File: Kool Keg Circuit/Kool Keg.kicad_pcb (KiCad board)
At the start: 2 copper layers, 84 parts, among them J1 Power, J2 Scale Header, J3 IR Header, J4 Flowmeter, J5 OLED, J6 Solenoid Conn, J7 USB_B_Micro, Q1 2N3905, Q2 2N3906, Q3 BC818, Q4 BC818, SW1 SW, SW2 SW, SW3 SW, SW4 SW_Push, SW5 SW_EN, U1 LM1117-ADJ, U2 TPS562207, U3 74LVC3G14, U4 HX711, U5 24LC256, U6 MPQ6610GS, U7 CP2102N, U8 ESP32-WROOM-32D

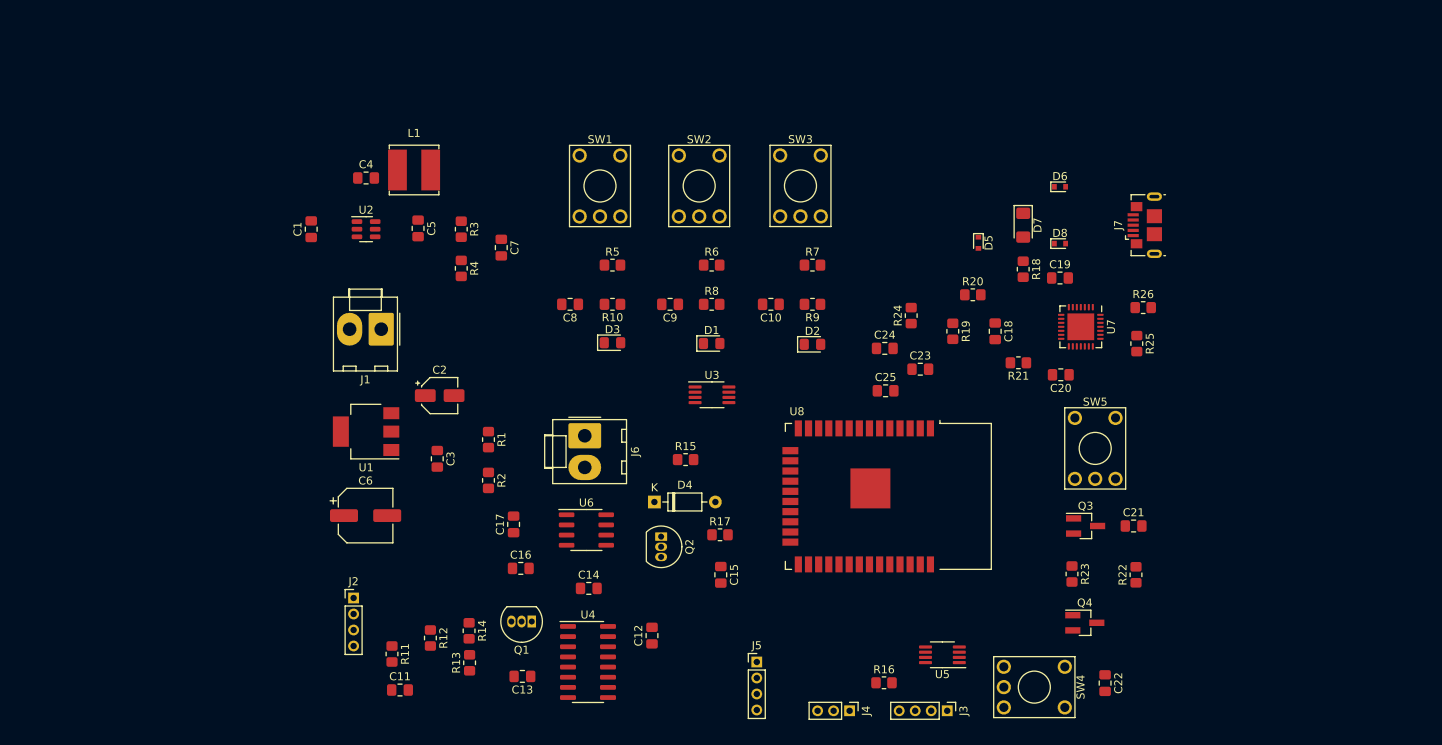
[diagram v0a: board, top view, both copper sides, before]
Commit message: PCB Layout
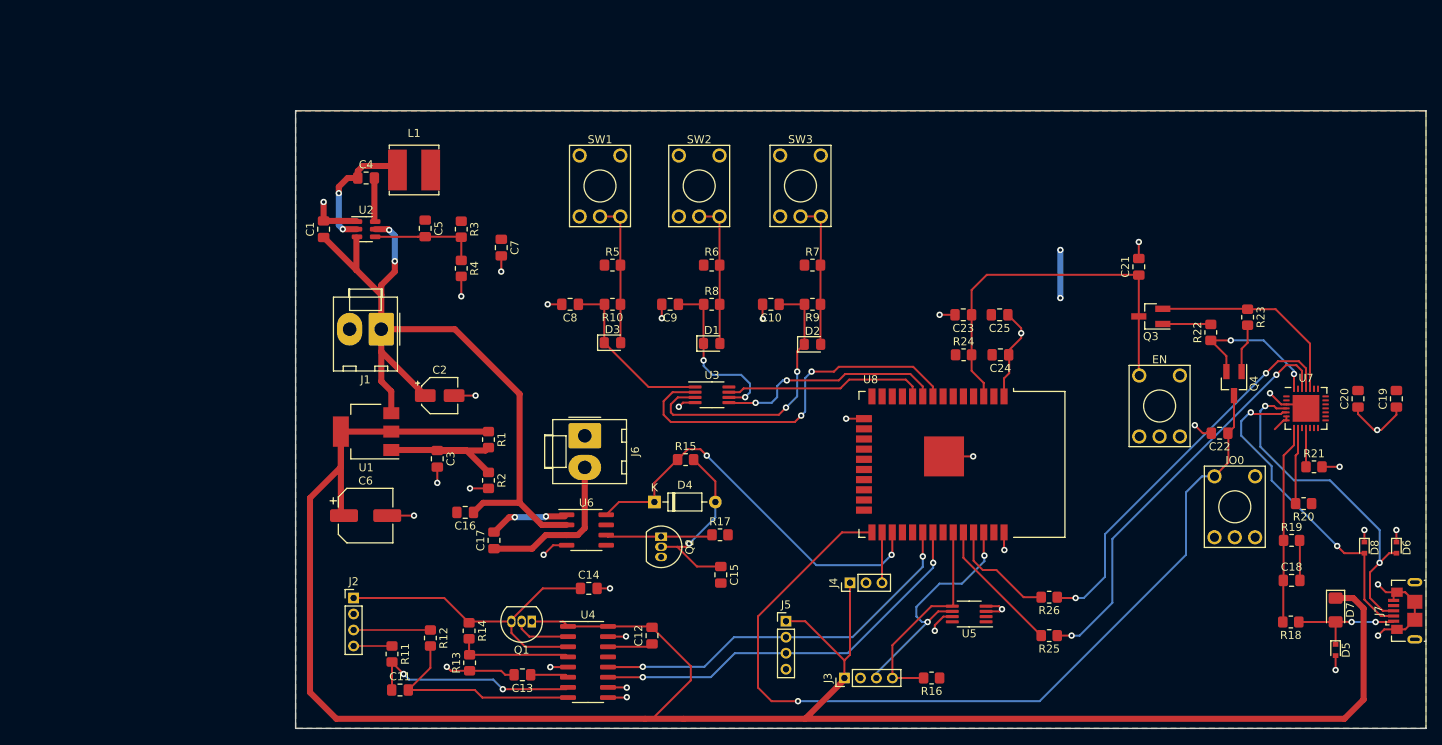
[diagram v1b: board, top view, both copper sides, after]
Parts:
- EN: renamed from SW5; value SW_EN -> SW_Push
- moved D5 67.7 mm to (225.7, 119.8)
- moved D7 62.0 mm to (225.7, 114.8)
- moved D6 61.7 mm to (233.3, 107.0), turned to -90 degrees
- moved J7 58.2 mm to (234.4, 114.9)
- moved R18 55.4 mm to (220.1, 116.3), turned to 180 degrees
- moved D8 53.8 mm to (229.3, 107.0), turned to -90 degrees
- moved R19 49.8 mm to (220.2, 106.1), turned to 0 degrees
- moved R20 48.9 mm to (221.7, 101.5), turned to 180 degrees
- moved C18 48.4 mm to (220.2, 111.1), turned to 0 degrees
- moved C19 44.7 mm to (233.3, 88.4), turned to 90 degrees
- moved R21 39.2 mm to (223.0, 96.9), turned to 0 degrees
- moved R23 38.9 mm to (214.7, 78.2)
- moved R25 38.1 mm to (189.9, 118.0), turned to 180 degrees
- moved R26 38.1 mm to (189.9, 113.2), turned to 180 degrees
- moved C20 37.3 mm to (228.5, 88.4), turned to 90 degrees
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- renumbered SW4 to IO0
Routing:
- net +5V: track 0.00 -> 273.8 mm
- net GND: track 0.00 -> 126.6 mm, vias 0 -> 35
- net /MCU Subsystem/IO0: track 0.00 -> 112.6 mm, vias 0 -> 1
- net +12V: track 0.00 -> 99.7 mm, vias 0 -> 2
- net /MCU Subsystem/TXD: track 0.00 -> 51.8 mm, vias 0 -> 2
- net /MCU Subsystem/I2C1_SCL: track 0.00 -> 50.7 mm, vias 0 -> 2
- net /MCU Subsystem/SOLENOID_GPIO: track 0.00 -> 49.9 mm, vias 0 -> 2
- net /MCU Subsystem/RXD: track 0.00 -> 49.4 mm, vias 0 -> 2
- net /MCU Subsystem/I2C1_SDA: track 0.00 -> 48.8 mm, vias 0 -> 2
- net /MCU Subsystem/EN: track 0.00 -> 48.2 mm
- net /MCU Subsystem/DEC: track 0.00 -> 47.7 mm, vias 0 -> 2
- net /MCU Subsystem/USB_DP: track 0.00 -> 42.5 mm, vias 0 -> 2
- net /MCU Subsystem/USB_DN: track 0.00 -> 40.9 mm, vias 0 -> 2
- net /Sensor Subsystem/E+: track 0.00 -> 40.0 mm
- net Net-(C10-Pad1): track 0.00 -> 36.3 mm, vias 0 -> 2
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- added copper zone on F.Cu, net +3.3V
- added copper zone on B.Cu, net GND
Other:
- board outline added: 141.3 x 77.2 mm

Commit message: PCB
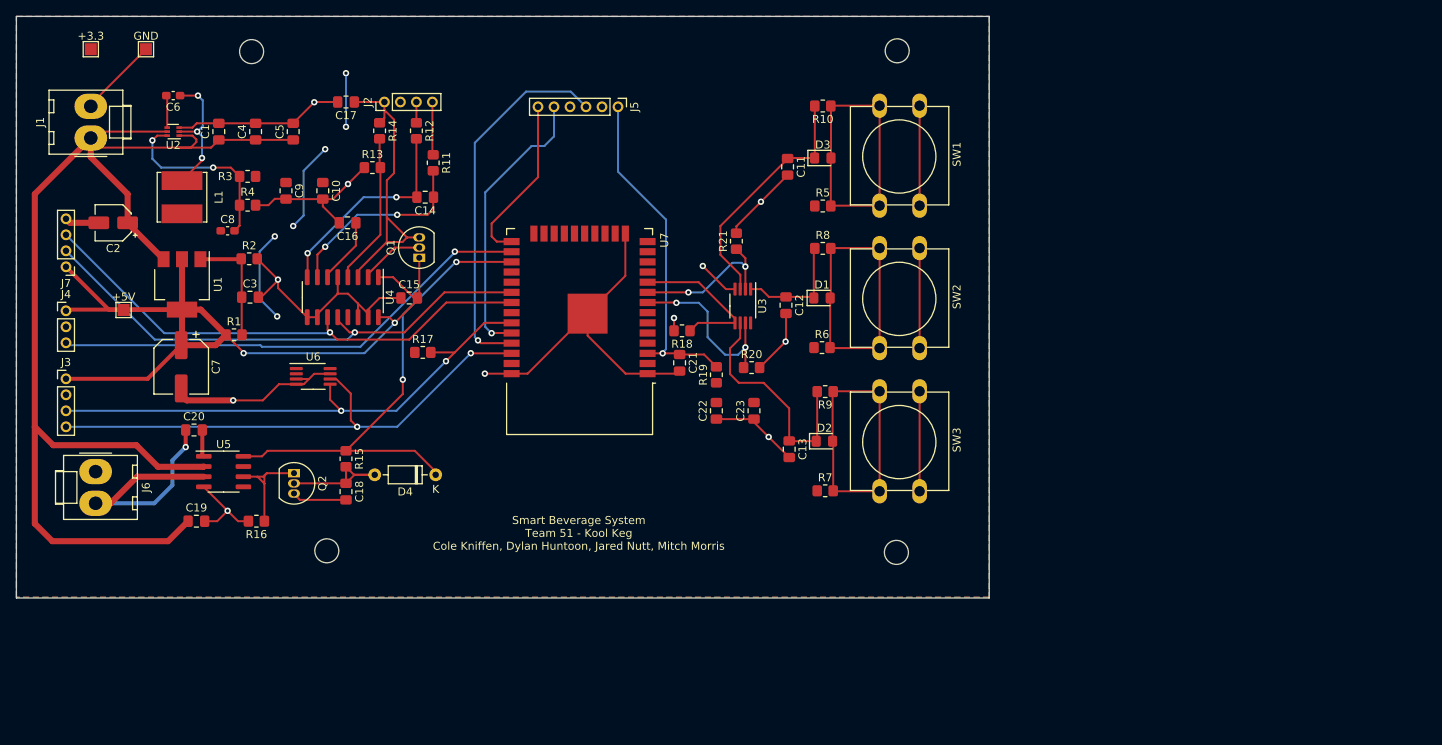
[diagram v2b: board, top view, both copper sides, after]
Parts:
- removed C24: 22uF, Capacitor_SMD:C_0805_2012Metric_Pad1.18x1.45mm_HandSolder
- removed C25: 0.1uF, Capacitor_SMD:C_0805_2012Metric_Pad1.18x1.45mm_HandSolder
- removed D5, D6, D8: LED, Diode_SMD:D_SOD-523
- removed D7: 1N5819, Diode_SMD:D_1206_3216Metric_Pad1.42x1.75mm_HandSolder
- removed EN, IO0: SW_Push, Button_Switch_THT:KSA_Tactile_SPST
- removed Q3, Q4: BC818, Package_TO_SOT_SMD:SOT-23_Handsoldering-BC808-25LT1g
- removed R22, R23, R24: 10k, Resistor_SMD:R_0805_2012Metric_Pad1.20x1.40mm_HandSolder
- removed R25, R26: 0R, Resistor_SMD:R_0805_2012Metric_Pad1.20x1.40mm_HandSolder
- removed U8: ESP32-WROOM-32D, RF_Module:ESP32-WROOM-32
- added +3.3: TestPoint_Pad_1.5x1.5mm, TestPoint:TestPoint_Pad_1.5x1.5mm, F.Cu at (70.1, 44.7)
- added +5V: TestPoint_Pad_1.5x1.5mm, TestPoint:TestPoint_Pad_1.5x1.5mm, F.Cu at (74.2, 77.3)
- added GND: TestPoint_Pad_1.5x1.5mm, TestPoint:TestPoint_Pad_1.5x1.5mm, F.Cu at (77.0, 44.7)
- added REF**: MountingHole_3mm, MountingHole:MountingHole_3mm, F.Cu at (99.6, 107.4)
- added REF**: MountingHole_3mm, MountingHole:MountingHole_3mm, F.Cu at (170.9, 44.9)
- added REF**: MountingHole_3mm, MountingHole:MountingHole_3mm, F.Cu at (170.8, 107.6)
- added REF**: MountingHole_3mm, MountingHole:MountingHole_3mm, F.Cu at (90.2, 45.0)
- C1: value 22uf -> 100nF
- C10, C9: value 0.1uF -> 22uF
- C12, C14: value 10uF -> 0.1uF
- C15: value 2.2uF -> 10uF
- C16: value .1uF -> 0.1uF
- C17: value 100 nF -> 10uF
- C18: value 10uF -> 2.2uF
- C19: value 4.7 uF -> .1uF
- C20: value 0.1 uF -> 100 nF
- C22: value 1n -> 22uF
- C23: value 1n -> 0.1uF
- C3: value 56nF -> 68nF
- C4: value .1uF -> 10uF
- C5: value 22pF -> 10uF
- C6: value 100uF -> .1uF; footprint Capacitor_SMD:CP_Elec_6.3x5.8 -> Capacitor_SMD:C_0603_1608Metric_Pad1.08x0.95mm_HandSolder
- C7: value 44uF -> 100uF; footprint Capacitor_SMD:C_0805_2012Metric_Pad1.18x1.45mm_HandSolder -> Capacitor_SMD:CP_Elec_6.3x5.8
- C8: value 0.1uF -> 56pF; footprint Capacitor_SMD:C_0805_2012Metric_Pad1.18x1.45mm_HandSolder -> Capacitor_SMD:C_0603_1608Metric_Pad1.08x0.95mm_HandSolder
- J3: value IR Header -> IR
- J4: value Flowmeter -> Flow
- J5: value OLED -> Prog; footprint Connector_PinHeader_2.00mm:PinHeader_1x04_P2.00mm_Vertical -> Connector_PinHeader_2.00mm:PinHeader_1x06_P2.00mm_Vertical
- J6: value Solenoid Conn -> Soloenoid
- J7: value USB_B_Micro -> OLED; footprint Connector_USB:USB_Micro-B_GCT_USB3076-30-A -> Connector_PinHeader_2.00mm:PinHeader_1x04_P2.00mm_Vertical
- R18: value 22.1k -> 10k
- R19: value 47.5k -> 10k
- R20: value 2k -> 10k
- SW1, SW2, SW3: value SW -> SW_MEC_5G; footprint Button_Switch_THT:KSA_Tactile_SPST -> Button_Switch_THT:SW_PUSH-12mm
- U2: footprint Package_TO_SOT_SMD:SOT-23-6 -> Package_TO_SOT_SMD:SOT-563
- U5: value 24LC256 -> 946-MPQ6610GS-AEC1-P; footprint Package_SO:MSOP-8_3x3mm_P0.65mm -> Package_SO:SOIC-8_3.9x4.9mm_P1.27mm
- U6: value MPQ6610GS -> 24LC256-I/MS; footprint Package_SO:SOIC-8_3.9x4.9mm_P1.27mm -> Package_SO:MSOP-8_3x3mm_P0.65mm
- U7: value CP2102N -> ESP32-WROOM-32D; footprint Package_DFN_QFN:QFN-28-1EP_5x5mm_P0.5mm_EP3.35x3.35mm -> RF_Module:ESP32-WROOM-32
- moved J7 172.8 mm to (67.0, 71.9), turned to 180 degrees
- moved C19 150.8 mm to (83.3, 103.7), turned to 0 degrees
- moved C20 145.6 mm to (83.0, 92.3), turned to 0 degrees
- moved C18 118.7 mm to (102.0, 100.0), turned to -90 degrees
- moved J3 104.2 mm to (67.0, 85.9), turned to 0 degrees
- moved J4 103.7 mm to (67.0, 77.4), turned to 0 degrees
- moved U5 94.9 mm to (86.7, 97.5), turned to 0 degrees
- moved U7 91.7 mm to (131.2, 77.0), turned to 180 degrees
- moved R16 86.6 mm to (90.8, 103.7)
- moved R18 84.4 mm to (144.0, 79.9)
- moved C11 81.4 mm to (157.2, 59.4), turned to -90 degrees
- moved R21 77.5 mm to (150.8, 68.7), turned to 90 degrees
- moved R19 74.8 mm to (148.3, 85.4), turned to 90 degrees
- moved R20 71.1 mm to (152.7, 84.5), turned to 0 degrees
- moved J5 67.6 mm to (136.0, 51.9), turned to -90 degrees
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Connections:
- C10 pad 1: Net-(C10-Pad1) -> +3.3V
- C11 pad 2: Net-(C11-Pad2) -> GND
- C12 pad 1: GND -> Net-(C12-Pad1)
- C12 pad 2: +5V -> GND
- C14 pad 1: /Sensor Subsystem/E+ -> Net-(C14-Pad1)
- C14 pad 2: GND -> Net-(C14-Pad2)
- C15 pad 1: Net-(C15-Pad1) -> GND
- C15 pad 2: GND -> +5V
- C16 pad 1: +12V -> Net-(C16-Pad1)
- C17 pad 1: Net-(C17-Pad1) -> /Sensor Subsystem/E+
- C17 pad 2: Net-(C17-Pad2) -> GND
- C18 pad 2: Net-(C18-Pad2) -> GND
- C19 pad 1: GND -> +12V
- C19 pad 2: +3.3V -> GND
- C20 pad 1: GND -> Net-(C20-Pad1)
- C20 pad 2: +3.3V -> Net-(C20-Pad2)
- C22 pad 1: /MCU Subsystem/IO0 -> GND
- C22 pad 2: GND -> +3.3V
- C23 pad 1: /MCU Subsystem/EN -> GND
- C23 pad 2: GND -> +3.3V
- C4 pad 1: Net-(C4-Pad1) -> +12V
- C4 pad 2: Net-(C4-Pad2) -> GND
- C5 pad 1: +3.3V -> +12V
- C5 pad 2: Net-(C5-Pad2) -> GND
- C6 pad 1: +5V -> Net-(C6-Pad1)
- C6 pad 2: GND -> Net-(C6-Pad2)
- C7 pad 1: +3.3V -> +5V
- C8 pad 1: Net-(C8-Pad1) -> +3.3V
- C8 pad 2: GND -> Net-(C8-Pad2)
- C9 pad 1: Net-(C9-Pad1) -> +3.3V
- D1 pad 1: Net-(C9-Pad1) -> Net-(C12-Pad1)
- D2 pad 1: Net-(C10-Pad1) -> Net-(C13-Pad1)
- D3 pad 1: Net-(C8-Pad1) -> Net-(C11-Pad1)
- D4 pad 2: Net-(C15-Pad1) -> Net-(C18-Pad1)
- J3 pad 3: /MCU Subsystem/I2C0_SCL -> /MCU Subsystem/I2C0_SDA
- J3 pad 4: /MCU Subsystem/I2C0_SDA -> /MCU Subsystem/I2C0_SCL
- J5 pad 1: +5V -> /MCU Subsystem/EN
- J5 pad 2: /MCU Subsystem/I2C1_SDA -> +3.3V
- J5 pad 3: /MCU Subsystem/I2C1_SCL -> /MCU Subsystem/TXD0
- J6 pad 2: Net-(C17-Pad1) -> Net-(C20-Pad1)
- J7 pad 1: /MCU Subsystem/VBUS -> +5V
- J7 pad 2: /MCU Subsystem/USB_DN -> /MCU Subsystem/I2C1_SDA
- J7 pad 3: /MCU Subsystem/USB_DP -> /MCU Subsystem/I2C1_SCL
- J7 pad 4: unconnected-(J7-Pad4) -> GND
- L1 pad 1: Net-(C4-Pad1) -> Net-(C6-Pad1)
- Q2 pad 2: Net-(C15-Pad1) -> Net-(C18-Pad1)
- R10 pad 2: Net-(C8-Pad1) -> Net-(C11-Pad1)
- R11 pad 2: Net-(C11-Pad1) -> Net-(C14-Pad1)
- R12 pad 2: Net-(C11-Pad2) -> Net-(C14-Pad2)
- R15 pad 2: Net-(C15-Pad1) -> Net-(C18-Pad1)
- R16 pad 1: +3.3V -> Net-(Q2-Pad1)
- R16 pad 2: /MCU Subsystem/I2C0_SDA -> GND
- R17 pad 1: Net-(Q2-Pad1) -> +3.3V
- R17 pad 2: GND -> /MCU Subsystem/I2C0_SDA
- R18 pad 1: /MCU Subsystem/VBUS -> /MCU Subsystem/DISP
- R18 pad 2: Net-(C18-Pad1) -> GND
- R19 pad 1: Net-(C18-Pad1) -> +3.3V
- R19 pad 2: Net-(C18-Pad2) -> /MCU Subsystem/EN
- R20 pad 1: +3.3V -> /MCU Subsystem/DEC
- R20 pad 2: Net-(R20-Pad2) -> GND
- R21 pad 1: Net-(R21-Pad1) -> /MCU Subsystem/INC
- R3 pad 2: Net-(C5-Pad2) -> Net-(C8-Pad2)
- R4 pad 1: Net-(C5-Pad2) -> Net-(C8-Pad2)
- R8 pad 1: Net-(C9-Pad1) -> Net-(C12-Pad1)
- R9 pad 2: Net-(C10-Pad1) -> Net-(C13-Pad1)
- SW1 pad 2: GND -> Net-(D3-Pad2)
- SW2 pad 2: GND -> Net-(D1-Pad2)
- SW3 pad 2: GND -> Net-(D2-Pad2)
- U2 pad 1: GND -> +12V
- U2 pad 2: Net-(C4-Pad1) -> Net-(C6-Pad1)
- U2 pad 3: +12V -> GND
- U2 pad 4: Net-(C5-Pad2) -> Net-(C6-Pad2)
- U2 pad 6: Net-(C4-Pad2) -> Net-(C8-Pad2)
- U3 pad 1: Net-(C8-Pad1) -> Net-(C12-Pad1)
- U3 pad 2: /MCU Subsystem/DEC -> /MCU Subsystem/INC
- U3 pad 3: Net-(C10-Pad1) -> Net-(C11-Pad1)
- U3 pad 5: /MCU Subsystem/INC -> /MCU Subsystem/DISP
- U3 pad 6: Net-(C9-Pad1) -> Net-(C13-Pad1)
- U3 pad 7: /MCU Subsystem/DISP -> /MCU Subsystem/DEC
- U4 pad 6: Net-(C13-Pad1) -> Net-(C16-Pad1)
- U4 pad 7: Net-(C11-Pad1) -> Net-(C14-Pad1)
- U4 pad 8: Net-(C11-Pad2) -> Net-(C14-Pad2)
- U5 pad 1: unconnected-(U5-Pad1) -> Net-(C20-Pad2)
- U5 pad 2: unconnected-(U5-Pad2) -> +12V
- U5 pad 3: GND -> Net-(C20-Pad1)
- U5 pad 5: /MCU Subsystem/I2C0_SDA -> unconnected-(U5-Pad5)
- U5 pad 6: /MCU Subsystem/I2C0_SCL -> Net-(Q2-Pad1)
- U5 pad 7: GND -> +3.3V
- U5 pad 8: +3.3V -> /MCU Subsystem/SOLENOID_GPIO
- U6 pad 1: Net-(C17-Pad2) -> unconnected-(U6-Pad1)
- U6 pad 2: +12V -> unconnected-(U6-Pad2)
- U6 pad 3: Net-(C17-Pad1) -> GND
- U6 pad 5: unconnected-(U6-Pad5) -> /MCU Subsystem/I2C0_SDA
- U6 pad 6: Net-(Q2-Pad1) -> /MCU Subsystem/I2C0_SCL
- U6 pad 7: +3.3V -> GND
- U6 pad 8: /MCU Subsystem/SOLENOID_GPIO -> +3.3V
- U7 pad 1: unconnected-(U7-Pad1) -> GND
- U7 pad 10: unconnected-(U7-Pad10) -> /MCU Subsystem/DISP
- U7 pad 11: Net-(R21-Pad1) -> unconnected-(U7-Pad11)
- U7 pad 15: unconnected-(U7-Pad15) -> GND
- U7 pad 2: unconnected-(U7-Pad2) -> +3.3V
- U7 pad 24: /MCU Subsystem/RTS -> unconnected-(U7-Pad24)
- U7 pad 25: /MCU Subsystem/RXD -> /MCU Subsystem/IO0
- U7 pad 26: /MCU Subsystem/TXD -> /MCU Subsystem/FLOW_GPIO
- U7 pad 27: unconnected-(U7-Pad27) -> /MCU Subsystem/SOLENOID_GPIO
- U7 pad 28: /MCU Subsystem/DTR -> unconnected-(U7-Pad28)
- U7 pad 29: GND -> unconnected-(U7-Pad29)
- U7 pad 3: GND -> /MCU Subsystem/EN
- U7 pad 4: /MCU Subsystem/USB_DP -> unconnected-(U7-Pad4)
- U7 pad 5: /MCU Subsystem/USB_DN -> unconnected-(U7-Pad5)
- U7 pad 6: +3.3V -> unconnected-(U7-Pad6)
- U7 pad 7: +3.3V -> unconnected-(U7-Pad7)
- U7 pad 8: Net-(C18-Pad1) -> /MCU Subsystem/DEC
- U7 pad 9: Net-(R20-Pad2) -> /MCU Subsystem/INC
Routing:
- net +5V: track 273.8 -> 112.5 mm, vias 0 -> 2
- net GND: track 126.6 -> 246.1 mm, vias 35 -> 11
- net /MCU Subsystem/IO0: track 112.6 -> 21.4 mm, vias 1 -> 0
- net +12V: track 99.7 -> 155.9 mm, vias 2 -> 0
- net /MCU Subsystem/FLOW_GPIO: track 6.31 -> 60.9 mm, vias 0 -> 1
- net /MCU Subsystem/TXD: track 51.8 -> 0.00 mm, vias 2 -> 0
- net /MCU Subsystem/RXD: track 49.4 -> 0.00 mm, vias 2 -> 0
- net /MCU Subsystem/USB_DP: track 42.5 -> 0.00 mm, vias 2 -> 0
- net /MCU Subsystem/USB_DN: track 40.9 -> 0.00 mm, vias 2 -> 0
- net /MCU Subsystem/I2C0_SDA: track 26.8 -> 67.2 mm, vias 0 -> 2
- net /MCU Subsystem/I2C0_SCL: track 30.7 -> 67.3 mm
- net Net-(C10-Pad1): track 36.3 -> 0.00 mm, vias 2 -> 0
- net Net-(C20-Pad1): track 0.00 -> 33.0 mm, vias 0 -> 1
- net /MCU Subsystem/TXD0: track 13.9 -> 46.5 mm, vias 0 -> 1
- net Net-(C11-Pad2): track 27.0 -> 0.00 mm
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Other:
- board size 141.3 x 77.2 mm -> 121.6 x 72.7 mm
- board text added: "Smart Beverage System Team 51 - Kool Keg Cole Kniffen, Dylan Huntoon, Jared Nutt, Mitch Morris"
